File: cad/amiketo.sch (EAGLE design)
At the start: 57 parts, among them CN1 MICROSD-EJECT, J1 HEADER-5X1, Q1 IRLML6344TRPBF, Q2 DMP2035U-7, SW2 SWITCHKMR211, SW3 SWITCHKMR211, U1 STM32F411/48, U2 LIS3DH, U3 ADP5062, U4 MCP1824, U5 MAX17048, X1 12MHz, X2 32k768

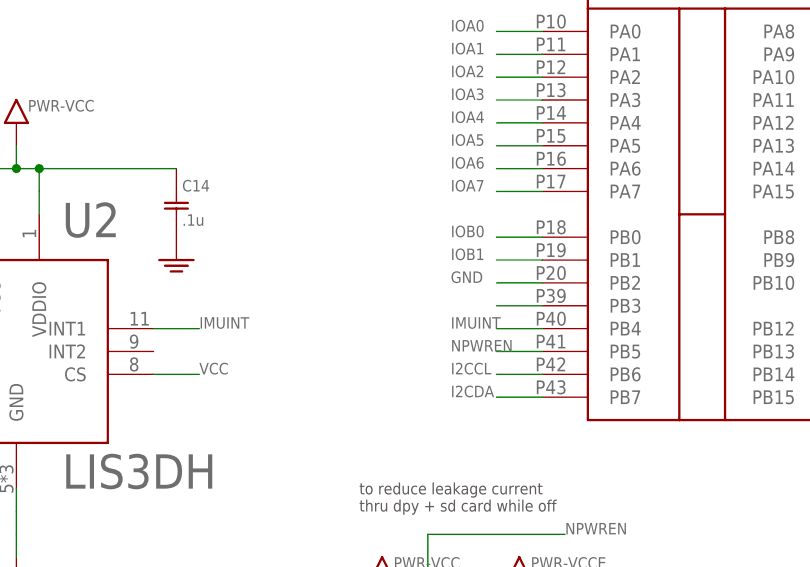
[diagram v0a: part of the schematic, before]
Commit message: i2c r, tweak
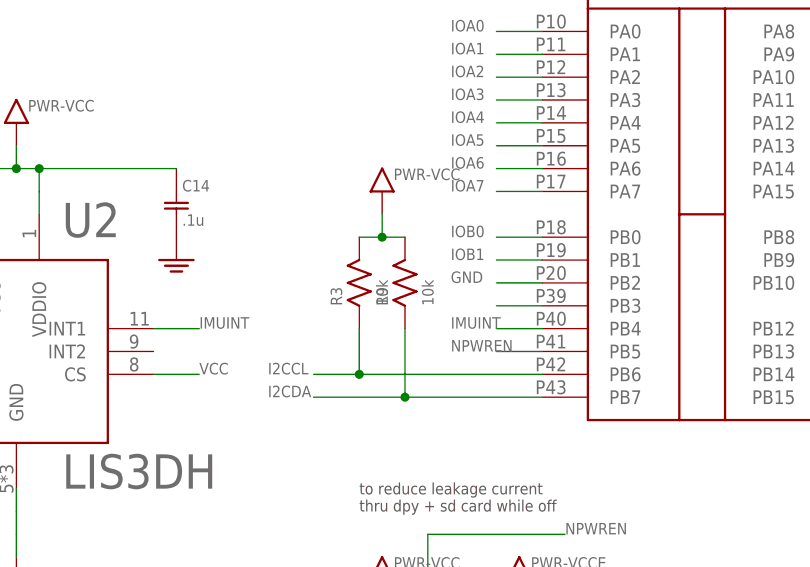
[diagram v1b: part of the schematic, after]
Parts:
- added R3, R9: 10k, jaw:R0603
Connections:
- net I2CCL: now also R3.P$1
- net I2CDA: now also R9.P$1
- net VCC: now also R3.P$2, R9.P$2
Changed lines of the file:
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@@
 <setting verticaltext="up"/>
 </settings>
-<grid distance="0.1" unitdist="inch" unit="inch" style="lines" multiple="1" display="yes" altdistance="0.01" altunitdist="inch" altunit="inch"/>
+<grid distance="0.1" unitdist="inch" unit="inch" style="lines" multiple="1" display="no" altdistance="0.01" altunitdist="inch" altunit="inch"/>
 <layers>
 <layer number="1" name="Top" color="4" fill="1" visible="no" active="no"/>
@@
 <part name="VCC6" library="jaw" deviceset="PWR-VCC" device=""/>
 <part name="D2" library="jaw" deviceset="DIODE" device="-0805" value="1A"/>
+<part name="R3" library="jaw" deviceset="R" device="0603" value="10k"/>
+<part name="R9" library="jaw" deviceset="R" device="0603" value="10k"/>
+<part name="VCC7" library="jaw" deviceset="PWR-VCC" device=""/>
 </parts>
 <sheets>
@@
 <instance part="VCC6" gate="G$1" x="193.04" y="200.66"/>
 <instance part="D2" gate="G$1" x="58.42" y="182.88"/>
+<instance part="R3" gate="G$1" x="137.16" y="114.3" rot="R90"/>
+<instance part="R9" gate="G$1" x="142.24" y="114.3" rot="R90"/>
+<instance part="VCC7" gate="G$1" x="139.7" y="124.46"/>
 </instances>
 <busses>
@@
 <pinref part="VCC6" gate="G$1" pin="VCC"/>
 </segment>
+<segment>
+<pinref part="R3" gate="G$1" pin="P$2"/>
+<pinref part="R9" gate="G$1" pin="P$2"/>
+<wire x1="137.16" y1="119.38" x2="139.7" y2="119.38" width="0.1524" layer="91"/>
+<pinref part="VCC7" gate="G$1" pin="VCC"/>
+<wire x1="139.7" y1="119.38" x2="142.24" y2="119.38" width="0.1524" layer="91"/>
+<wire x1="139.7" y1="119.38" x2="139.7" y2="121.92" width="0.1524" layer="91"/>
+<junction x="139.7" y="119.38"/>
+</segment>
 </net>
 <net name="BOOT0" class="0">
@@
 <segment>
 <pinref part="U1" gate="G$1" pin="PB6"/>
-<wire x1="157.48" y1="104.14" x2="152.4" y2="104.14" width="0.1524" layer="91"/>
-<label x="147.32" y="104.14" size="1.27" layer="95"/>
+<wire x1="157.48" y1="104.14" x2="137.16" y2="104.14" width="0.1524" layer="91"/>
+<label x="127" y="104.14" size="1.27" layer="95"/>
+<pinref part="R3" gate="G$1" pin="P$1"/>
+<wire x1="137.16" y1="104.14" x2="132.08" y2="104.14" width="0.1524" layer="91"/>
+<wire x1="137.16" y1="109.22" x2="137.16" y2="104.14" width="0.1524" layer="91"/>
+<junction x="137.16" y="104.14"/>
 </segment>
 <segment>
@@
 <segment>
 <pinref part="U1" gate="G$1" pin="PB7"/>
-<wire x1="157.48" y1="101.6" x2="152.4" y2="101.6" width="0.1524" layer="91"/>
-<label x="147.32" y="101.6" size="1.27" layer="95"/>
-</segment>
-<segment>
+<wire x1="157.48" y1="101.6" x2="142.24" y2="101.6" width="0.1524" layer="91"/>
+<label x="127" y="101.6" size="1.27" layer="95"/>
+<pinref part="R9" gate="G$1" pin="P$1"/>
+<wire x1="142.24" y1="101.6" x2="132.08" y2="101.6" width="0.1524" layer="91"/>
+<wire x1="142.24" y1="109.22" x2="142.24" y2="101.6" width="0.1524" layer="91"/>
+<junction x="142.24" y="101.6"/>
+</segment>
+<segment>

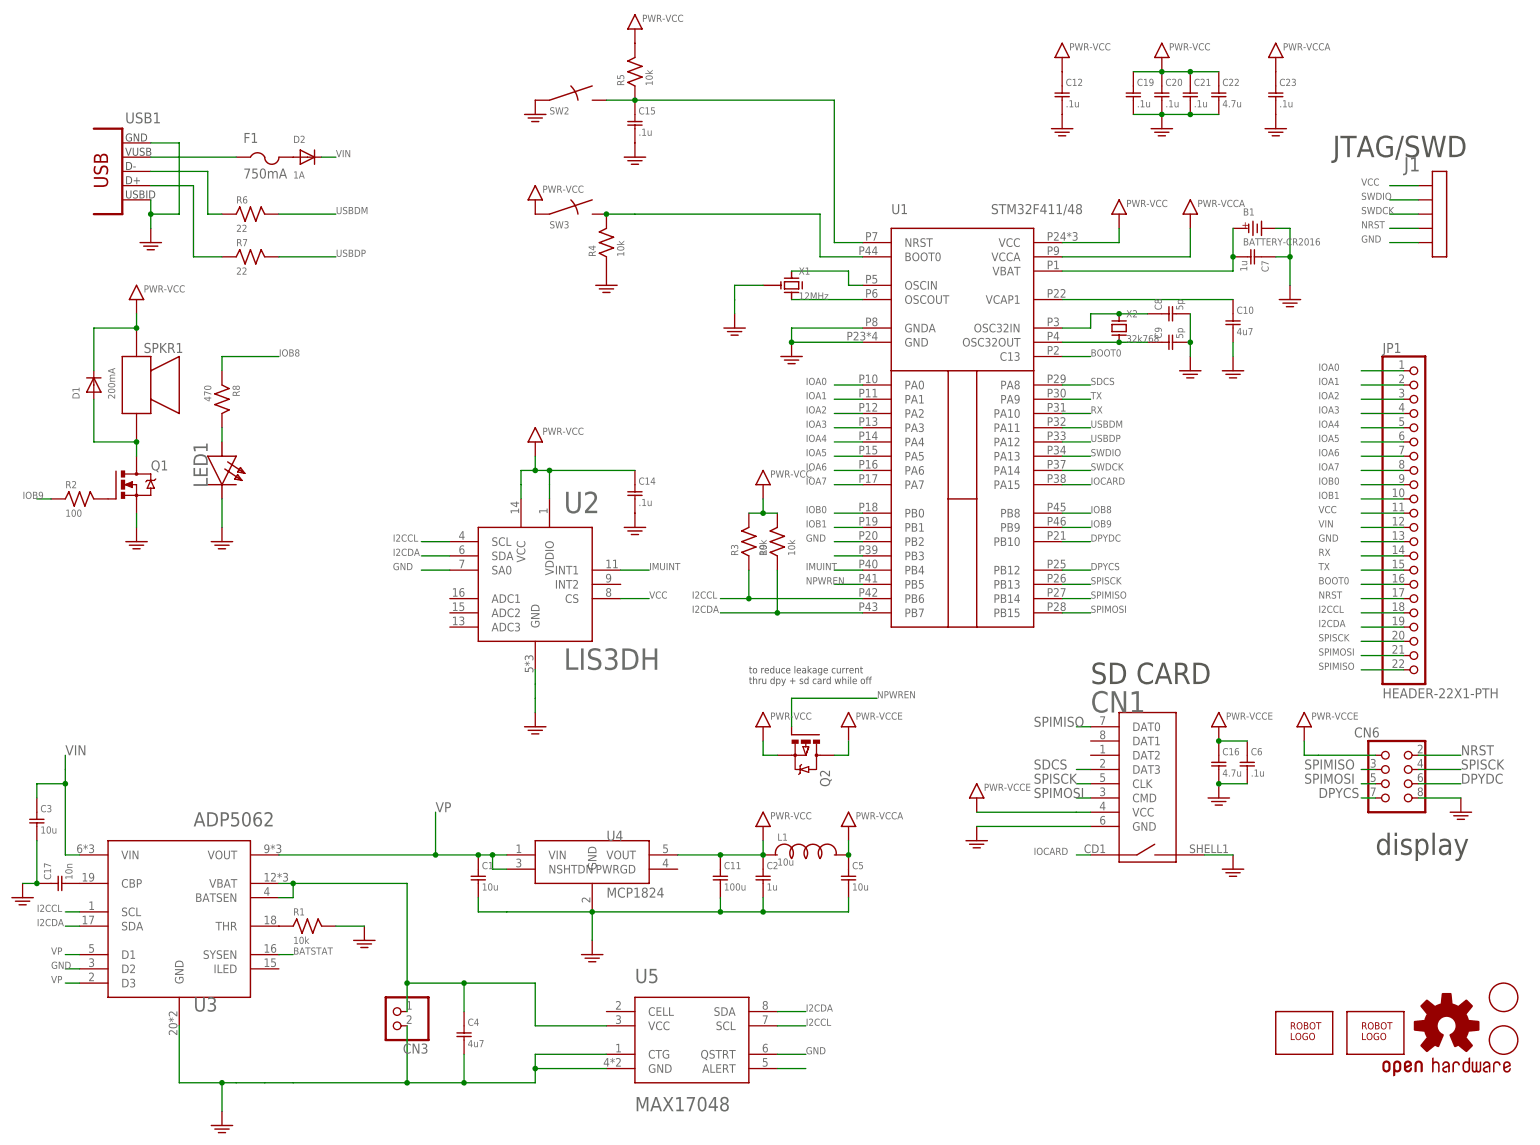
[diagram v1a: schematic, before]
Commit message: swap regulator
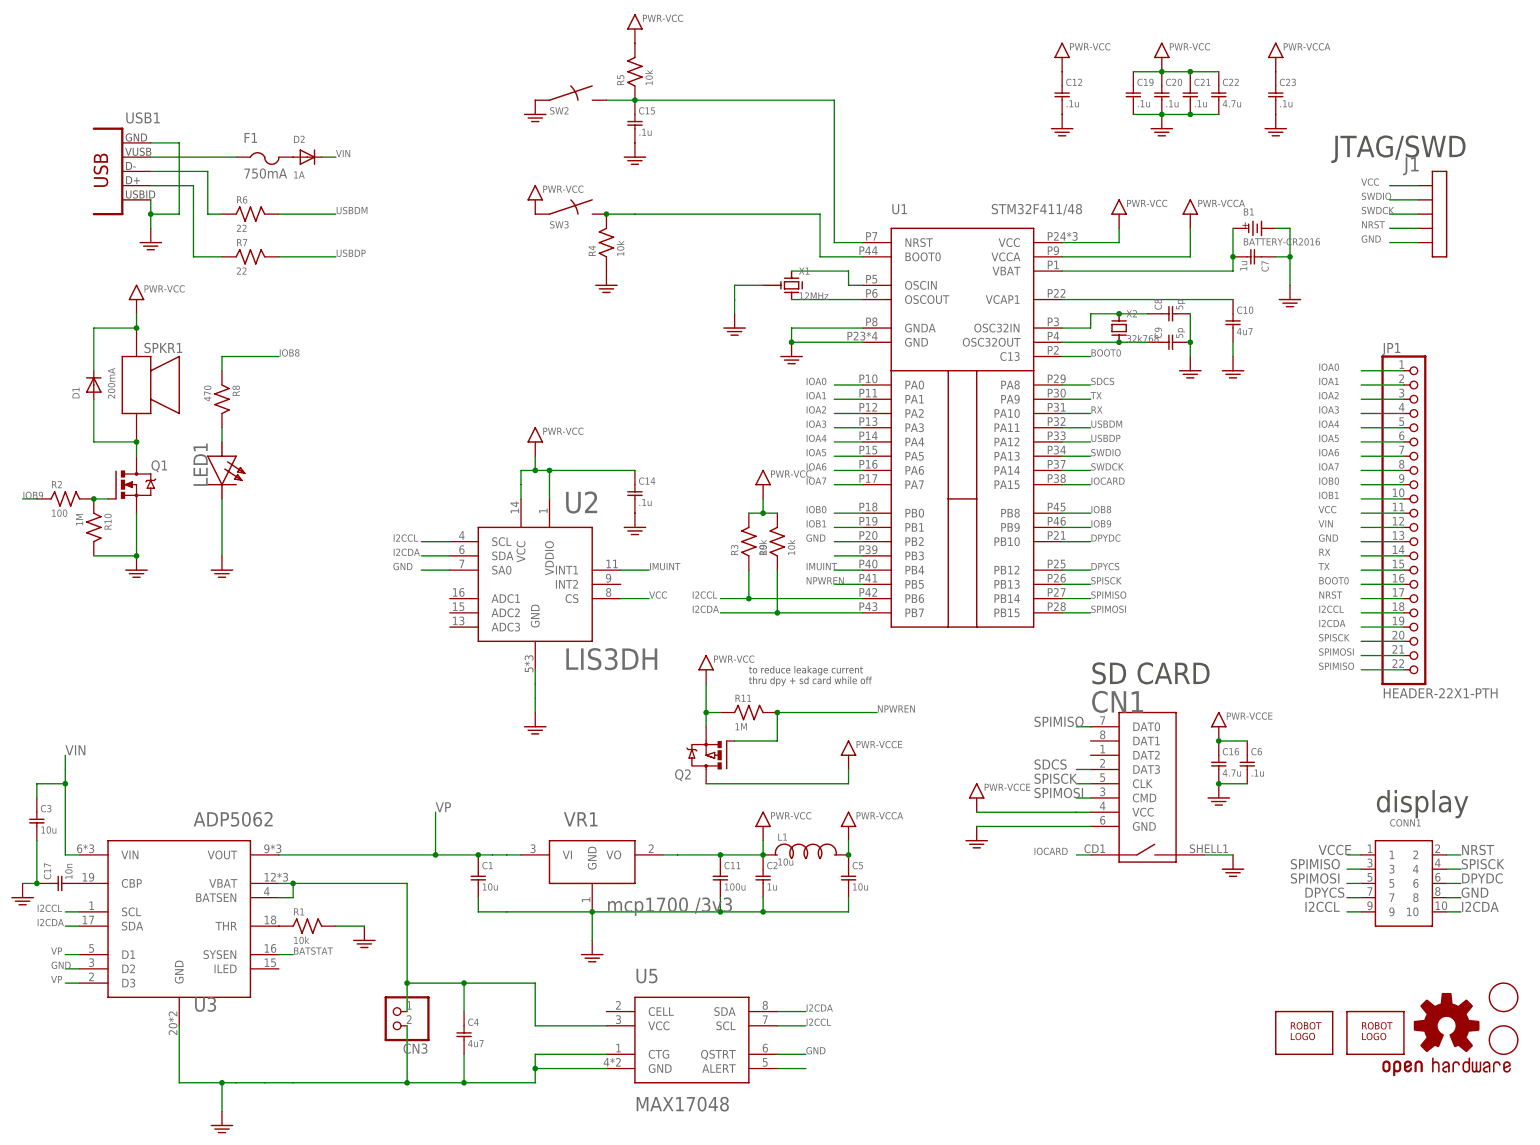
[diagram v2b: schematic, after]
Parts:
- removed CN6: (no value), jaw:HEADER-2X4
- removed U4: MCP1824, jaw:MCP1824
- added CONN1: HEADER-5X2-PTH, jaw:HEADER-5X2-PTH
- added R10, R11: 1M, jaw:R0603
- added VR1: mcp1700 /3v3, jaw:REGULATOR-SOT23-3
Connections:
- net DPYCS: now also CONN1.7; no longer CN6.P$7
- net DPYDC: now also CONN1.6; no longer CN6.P$6
- net GND: now also CONN1.8, R10.P$2, VR1.GND; no longer CN6.P$8, U4.GND
- net I2CCL: now also CONN1.9
- net I2CDA: now also CONN1.10
- net N$9: now also R10.P$1
- net NPWREN: now also R11.P$2
- net NRST: now also CONN1.2; no longer CN6.P$2
- net SPIMISO: now also CONN1.3; no longer CN6.P$3
- net SPIMOSI: now also CONN1.5; no longer CN6.P$5
- net SPISCK: now also CONN1.4; no longer CN6.P$4
- net VCC: now also R11.P$1, VR1.VO; no longer U4.VOUT
- net VCCE: now also CONN1.1; no longer CN6.P$1
- net VP: now also VR1.VI; no longer U4.NSHTDN, U4.VIN
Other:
- moved on the sheet: Q2, R2
